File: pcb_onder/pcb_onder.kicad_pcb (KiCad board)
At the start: 2 copper layers, 18 parts

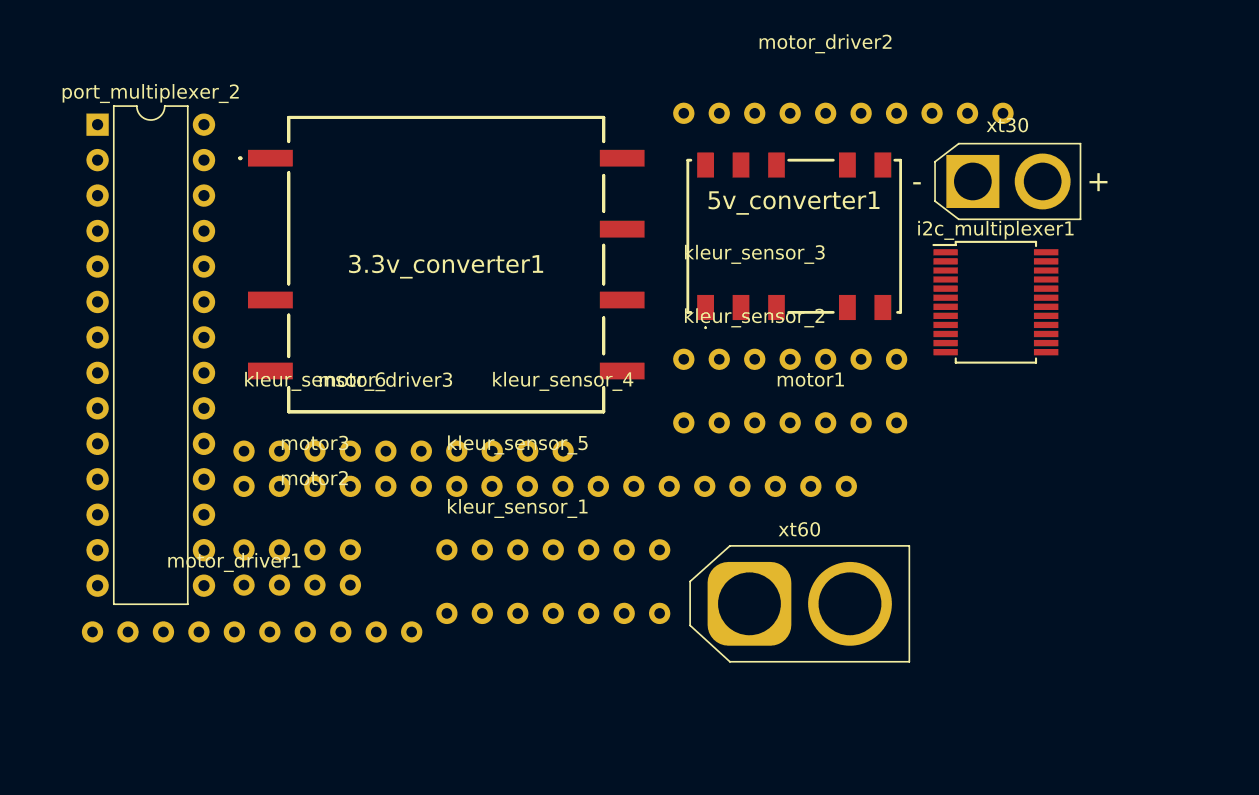
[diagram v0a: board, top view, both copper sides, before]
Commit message: pcb onder gemaakt
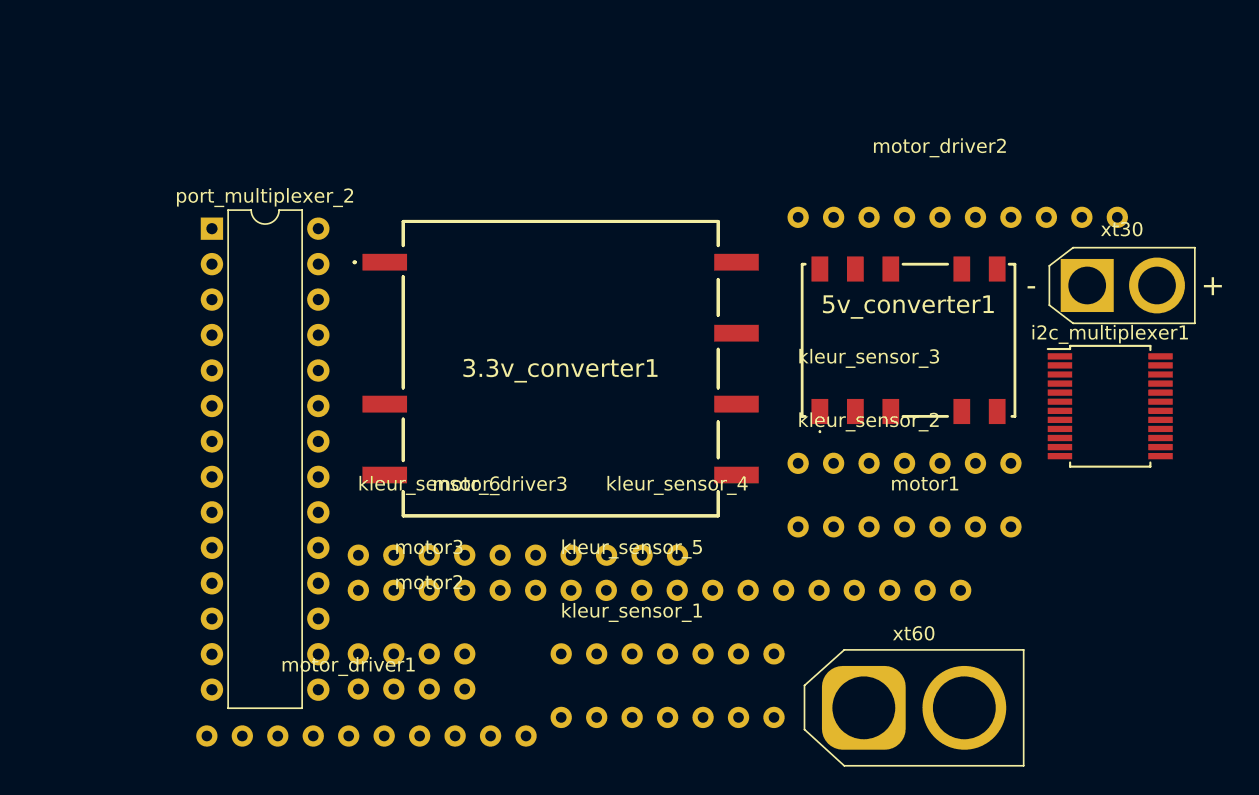
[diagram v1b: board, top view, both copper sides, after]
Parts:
- moved 3.3v_converter1 11.1 mm to (142.2, 104.1)
- moved 5v_converter1 11.1 mm to (167.2, 102.1)
- moved kleur_sensor_1 11.1 mm to (147.4, 131.7)
- moved kleur_sensor_2 11.1 mm to (164.3, 118.0)
- moved kleur_sensor_3 11.1 mm to (164.3, 113.5)
- moved kleur_sensor_4 11.1 mm to (150.6, 122.6)
- moved kleur_sensor_6 11.1 mm to (132.8, 122.6)
- moved motor2 11.1 mm to (132.8, 127.1)
- moved motor3 11.1 mm to (132.8, 124.6)
- moved motor_driver1 11.1 mm to (127.1, 130.5)
- moved xt30 11.1 mm to (180.0, 98.2)
- moved xt60 11.1 mm to (164.0, 128.4)
- moved i2c_multiplexer1 11.1 mm to (181.6, 106.8)
- moved kleur_sensor_5 11.1 mm to (147.4, 127.1)
- moved motor1 11.1 mm to (168.4, 120.0)
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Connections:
- 3.3v_converter1 pad 5: gnd -> Net-(3.3v_converter1-Pad5)
- i2c_multiplexer1 pad 12: gnd -> Net-(3.3v_converter1-Pad5)
- kleur_sensor_1 pad 3: gnd -> Net-(3.3v_converter1-Pad5)
- kleur_sensor_2 pad 3: gnd -> Net-(3.3v_converter1-Pad5)
- kleur_sensor_3 pad 3: gnd -> Net-(3.3v_converter1-Pad5)
- kleur_sensor_4 pad 3: gnd -> Net-(3.3v_converter1-Pad5)
- kleur_sensor_5 pad 3: gnd -> Net-(3.3v_converter1-Pad5)
- kleur_sensor_6 pad 3: gnd -> Net-(3.3v_converter1-Pad5)
- motor_driver1 pad 6: gnd -> Net-(3.3v_converter1-Pad5)
- motor_driver2 pad 6: gnd -> Net-(3.3v_converter1-Pad5)
- motor_driver3 pad 6: gnd -> Net-(3.3v_converter1-Pad5)
- port_multiplexer_2 pad 10: gnd -> Net-(3.3v_converter1-Pad5)
